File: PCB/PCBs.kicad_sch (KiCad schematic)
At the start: 12 parts, among them CN1 W2A41C681KAT2A, U1 ADS1299IPAGR, U4 TPD4E1B06DCKR

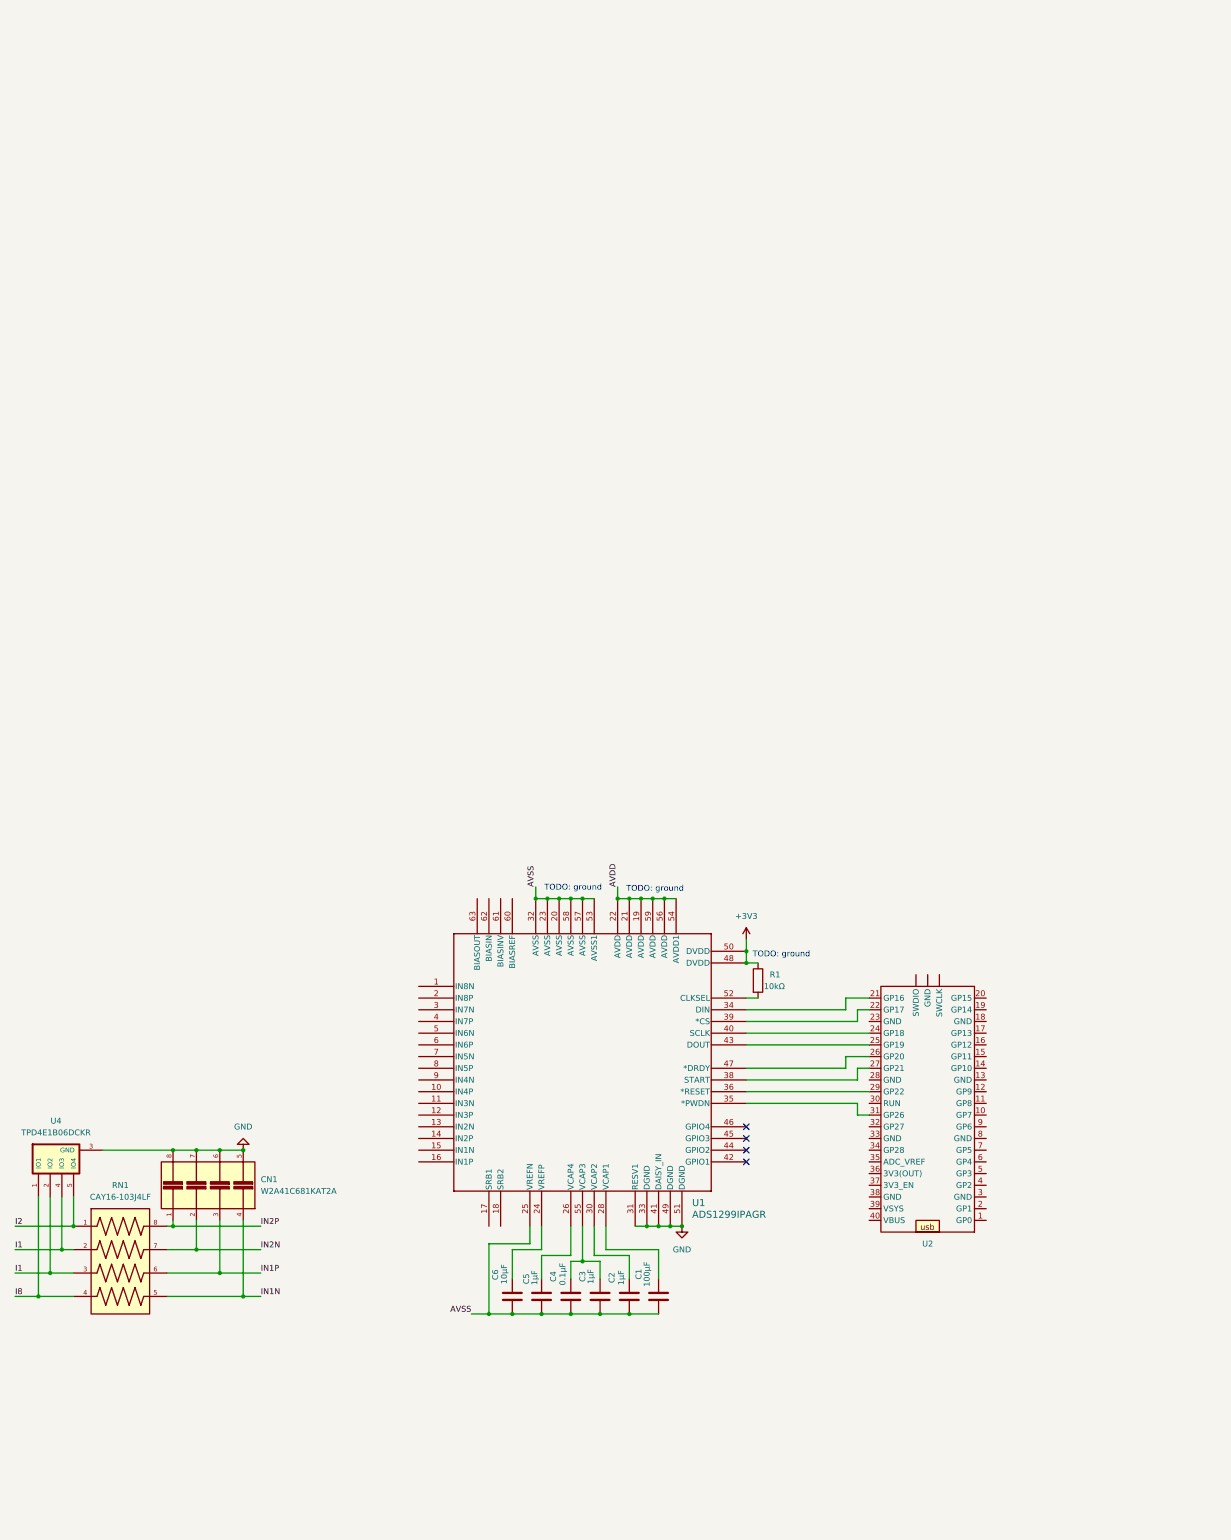
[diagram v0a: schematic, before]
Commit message: input cp
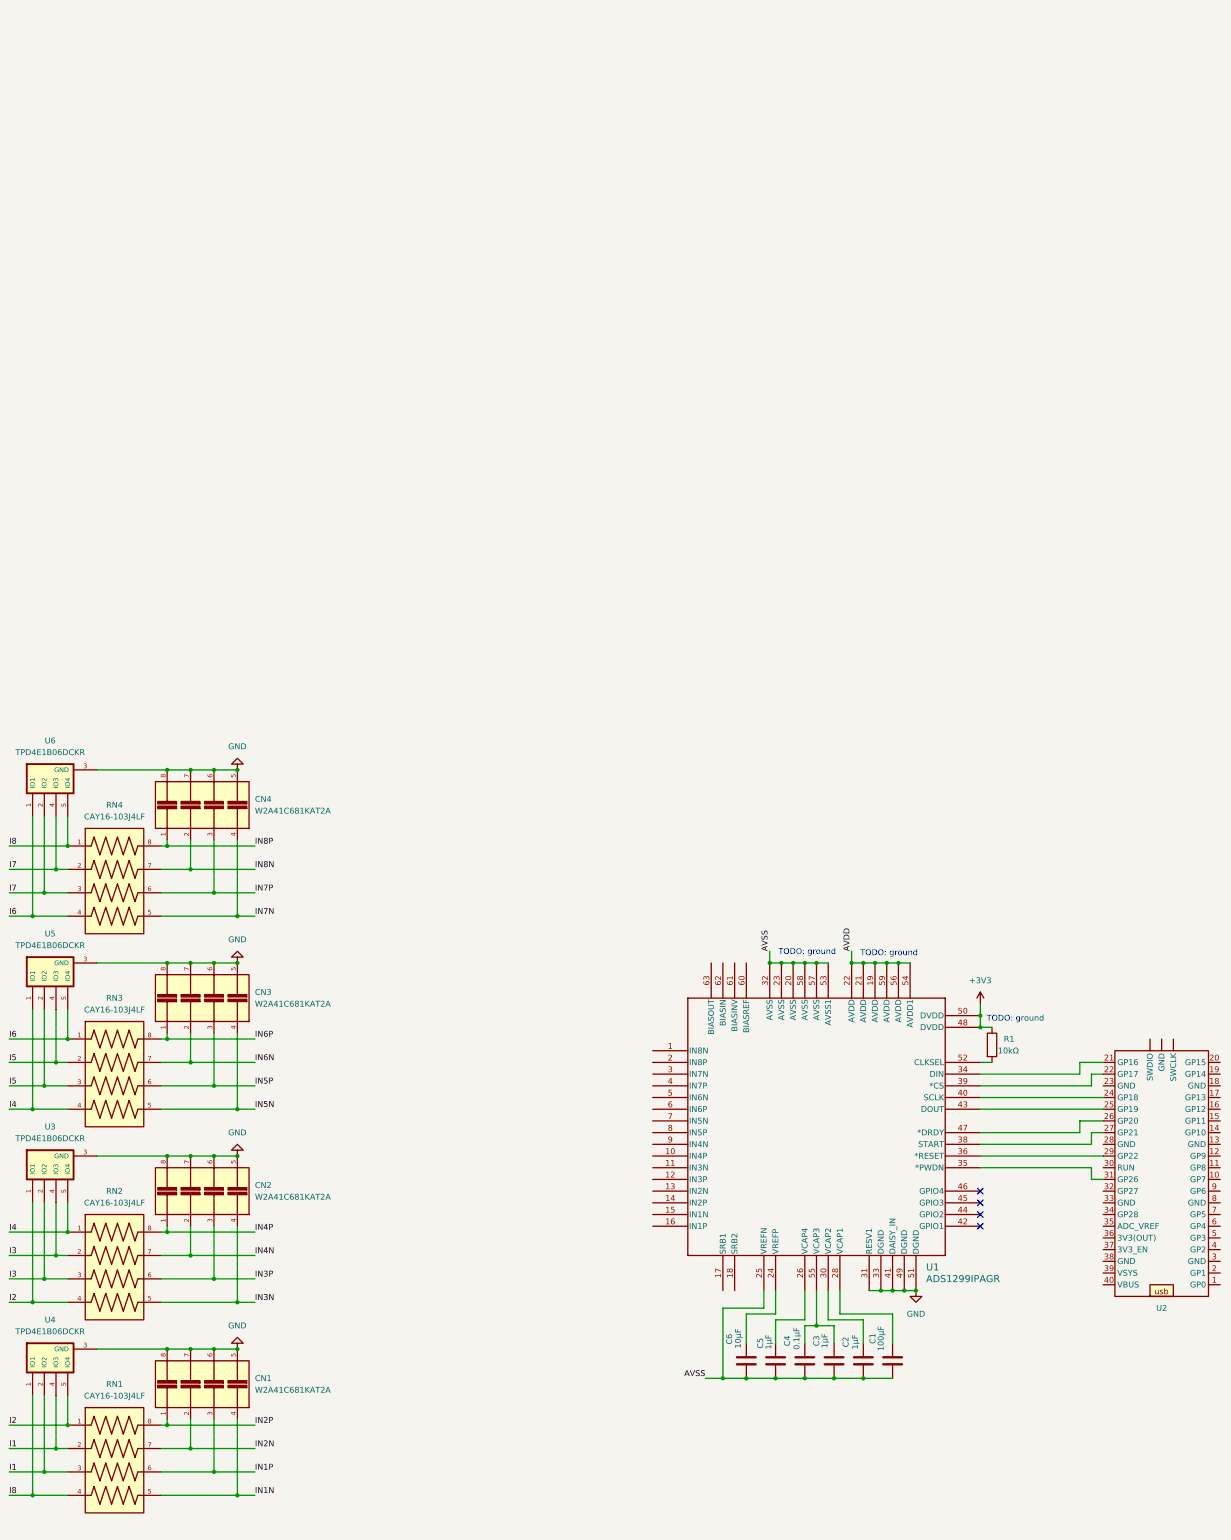
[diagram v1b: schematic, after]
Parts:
- added CN2, CN3, CN4: W2A41C681KAT2A, W2A41C681KAT2A:CAPCAXE50P210X130X94-8N, symbol custom_lib:W2A41C681KAT2A
- added RN2, RN3, RN4: CAY16-103J4LF, CAY16-103J4LF:RESCAF80P320X160X60-8N, symbol custom_lib:CAY16-103J4LF
- added U3, U5, U6: TPD4E1B06DCKR, TPD4E1B06DCKR:SOT65P210X110-6N, symbol custom_lib:TPD4E1B06DCKR
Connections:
- net GND: now also CN2.5, CN2.6, CN2.7, CN2.8, CN3.5, CN3.6, CN3.7, CN3.8, CN4.5, CN4.6, CN4.7, CN4.8, U3.3 (GND), U5.3 (GND), U6.3 (GND)
- net I2: now also RN2.4, U3.1 (IO1)
- net I8: now also RN4.1, U6.5 (IO4)
- new net I3: RN2.2, RN2.3, U3.2 (IO2), U3.4 (IO3)
- new net I4: RN2.1, RN3.4, U3.5 (IO4), U5.1 (IO1)
- new net I5: RN3.2, RN3.3, U5.2 (IO2), U5.4 (IO3)
- new net I6: RN3.1, RN4.4, U5.5 (IO4), U6.1 (IO1)
- new net I7: RN4.2, RN4.3, U6.2 (IO2), U6.4 (IO3)
- new net IN3N: CN2.4, RN2.5
- new net IN3P: CN2.3, RN2.6
- new net IN4N: CN2.2, RN2.7
- new net IN4P: CN2.1, RN2.8
- new net IN5N: CN3.4, RN3.5
- new net IN5P: CN3.3, RN3.6
- new net IN6N: CN3.2, RN3.7
- new net IN6P: CN3.1, RN3.8
- new net IN7N: CN4.4, RN4.5
- new net IN7P: CN4.3, RN4.6
- new net IN8N: CN4.2, RN4.7
- new net IN8P: CN4.1, RN4.8
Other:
- moved on the sheet: C1, C2, C3, C4, C5, C6, CN1, R1, RN1, U1, U2, U4

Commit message: input offset montage
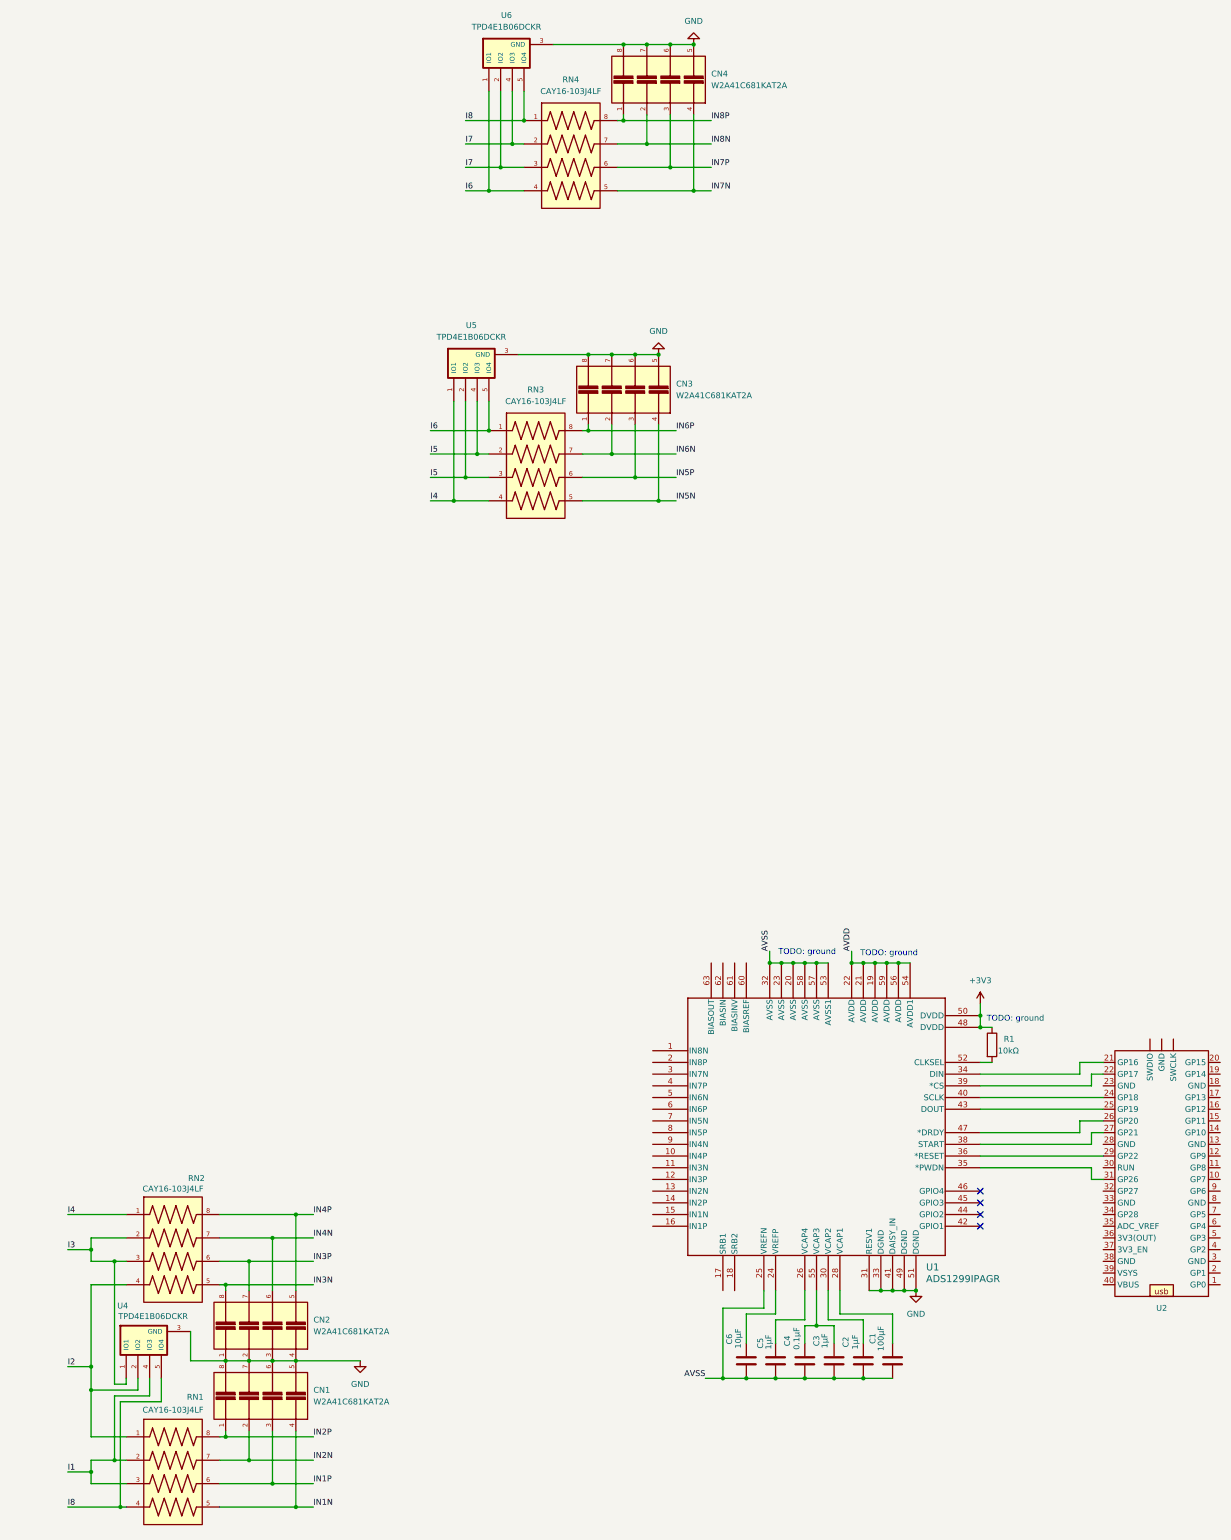
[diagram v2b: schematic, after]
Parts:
- removed U3: TPD4E1B06DCKR, TPD4E1B06DCKR:SOT65P210X110-6N, symbol custom_lib:TPD4E1B06DCKR
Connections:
- net GND: now also CN2.1, CN2.2, CN2.3, CN2.4; no longer CN2.5, CN2.6, CN2.7, CN2.8
- net I1: no longer U4.2 (IO2)
- net I2: now also U4.2 (IO2); no longer U4.5 (IO4)
- net I3: now also U4.1 (IO1)
- net I8: now also U4.5 (IO4); no longer U4.1 (IO1)
- net IN3N: now also CN2.8; no longer CN2.4
- net IN3P: now also CN2.7; no longer CN2.3
- net IN4N: now also CN2.6; no longer CN2.2
- net IN4P: now also CN2.5; no longer CN2.1
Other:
- moved on the sheet: CN1, CN2, CN3, CN4, RN1, RN2, RN3, RN4, U5, U6

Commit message: duplicate input
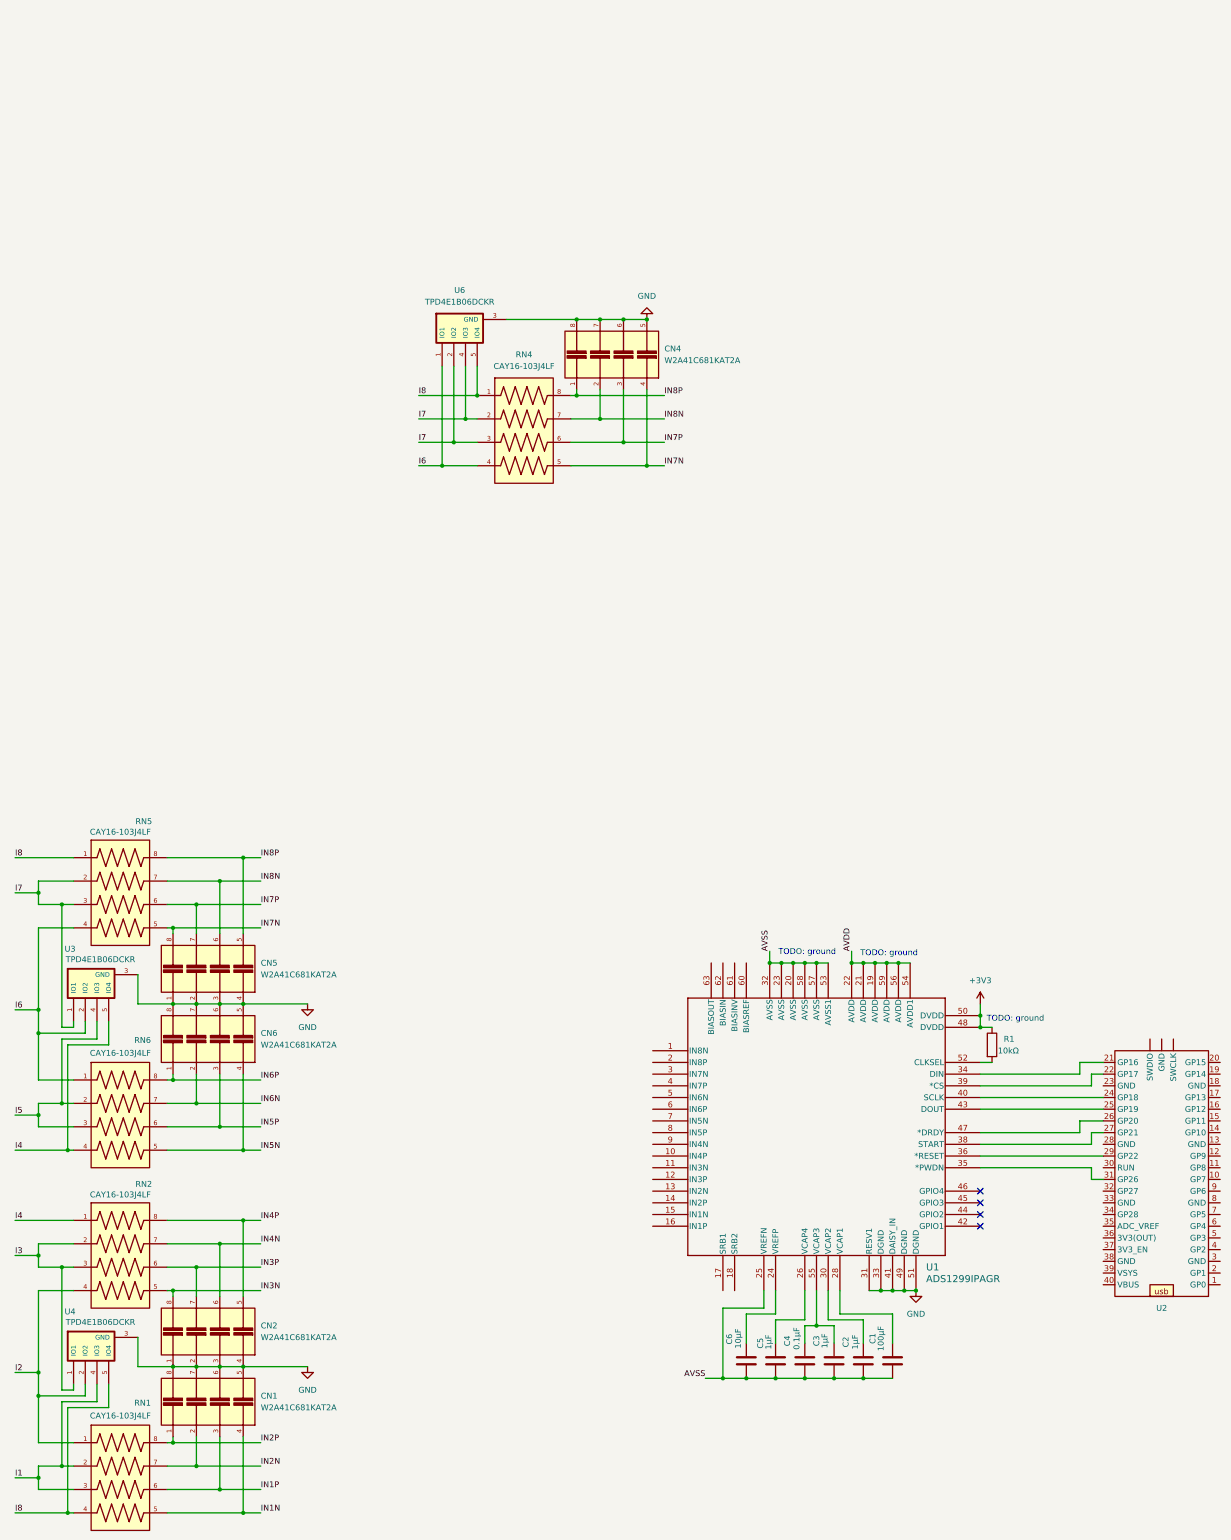
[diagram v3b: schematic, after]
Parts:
- removed CN3: W2A41C681KAT2A, W2A41C681KAT2A:CAPCAXE50P210X130X94-8N, symbol custom_lib:W2A41C681KAT2A
- removed RN3: CAY16-103J4LF, CAY16-103J4LF:RESCAF80P320X160X60-8N, symbol custom_lib:CAY16-103J4LF
- removed U5: TPD4E1B06DCKR, TPD4E1B06DCKR:SOT65P210X110-6N, symbol custom_lib:TPD4E1B06DCKR
- added CN5, CN6: W2A41C681KAT2A, W2A41C681KAT2A:CAPCAXE50P210X130X94-8N, symbol custom_lib:W2A41C681KAT2A
- added RN5, RN6: CAY16-103J4LF, CAY16-103J4LF:RESCAF80P320X160X60-8N, symbol custom_lib:CAY16-103J4LF
- added U3: TPD4E1B06DCKR, TPD4E1B06DCKR:SOT65P210X110-6N, symbol custom_lib:TPD4E1B06DCKR
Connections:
- net GND: now also CN5.1, CN5.2, CN5.3, CN5.4, CN6.5, CN6.6, CN6.7, CN6.8, U3.3 (GND)
- net I4: now also RN6.4, U3.5 (IO4)
- net I5: now also RN6.2, RN6.3, U3.4 (IO3)
- net I6: now also RN5.4, RN6.1, U3.2 (IO2)
- net I7: now also RN5.2, RN5.3, U3.1 (IO1)
- net I8: now also RN5.1
- net IN5N: now also CN6.4, RN6.5
- net IN5P: now also CN6.3, RN6.6
- net IN6N: now also CN6.2, RN6.7
- net IN6P: now also CN6.1, RN6.8
- net IN7N: now also CN5.8, RN5.5
- net IN7P: now also CN5.7, RN5.6
- net IN8N: now also CN5.6, RN5.7
- net IN8P: now also CN5.5, RN5.8
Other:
- moved on the sheet: CN1, CN2, CN4, RN1, RN2, RN4, U4, U6
